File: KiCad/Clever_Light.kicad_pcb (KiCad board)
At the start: 2 copper layers, 50.8 x 50.8 mm, 18 parts, among them IC1 BTA08-600SWRG, J1 Screw_Terminal_01x02, J2 Screw_Terminal_01x02, J3 Screw_Terminal_01x02, J4 Screw_Terminal_01x02, J5 Conn_02x07_Odd_Even, Q1 SFH6156-3T, U1 MOC3063M

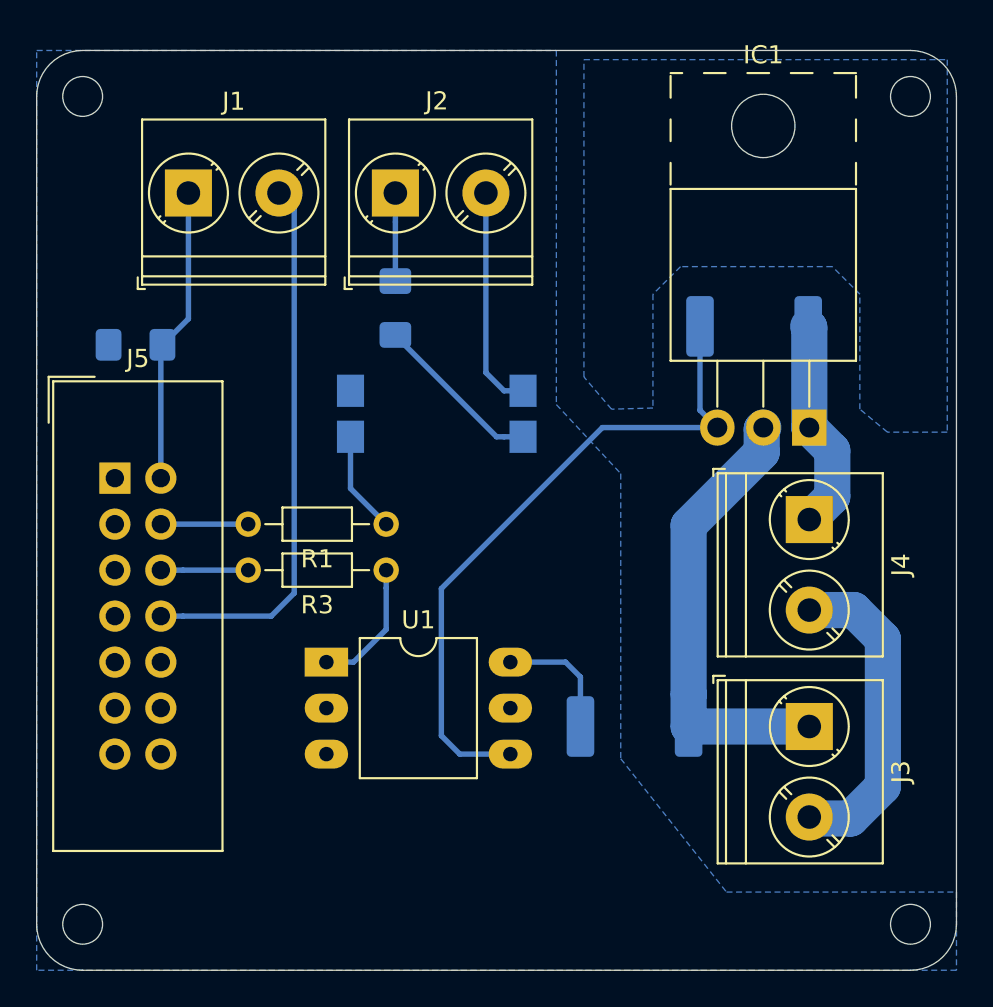
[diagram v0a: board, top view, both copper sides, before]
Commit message: небольшая оптимизация
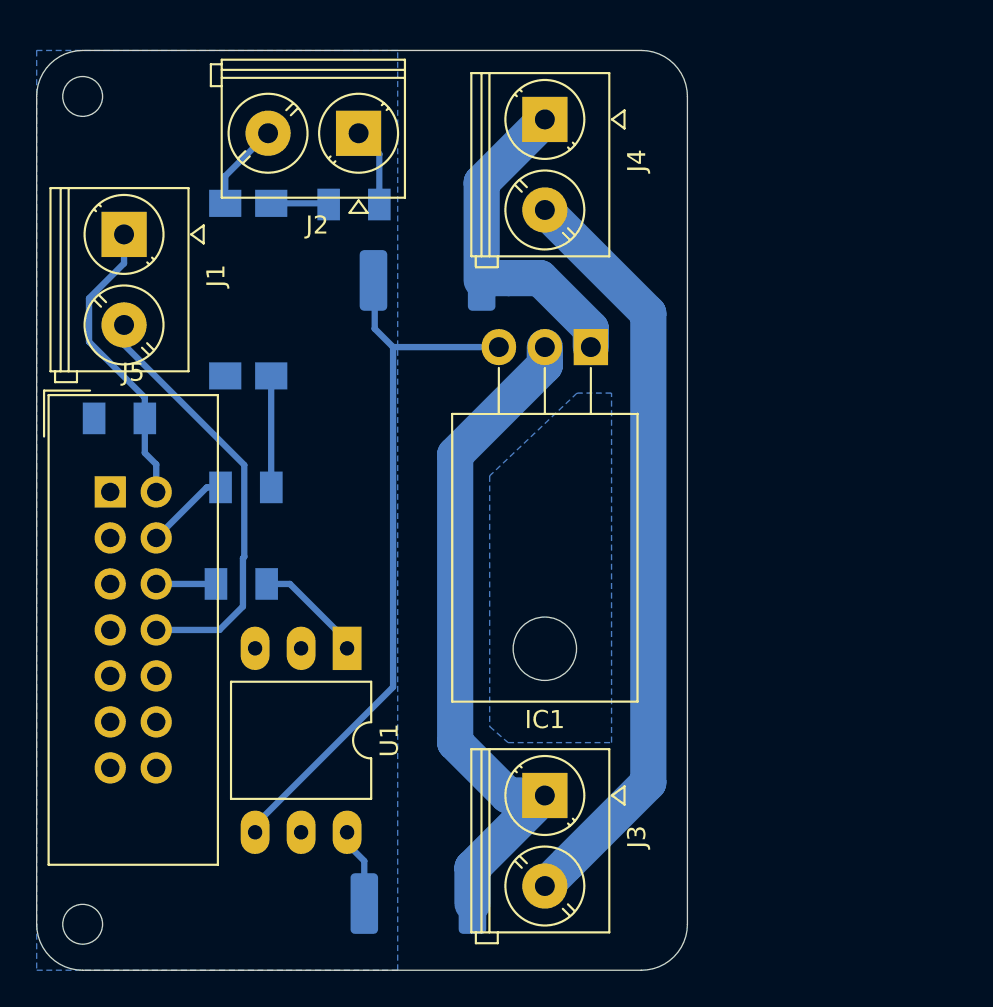
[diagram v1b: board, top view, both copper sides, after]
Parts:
- removed the REF** at (159.3, 93.2)
- removed the REF** at (159.3, 47.5)
- IC1: footprint Package_TO_SOT_THT:TO-220-3_Horizontal_TabUp -> Package_TO_SOT_THT:TO-220-3_Horizontal_TabDown
- J1, J2, J3, J4: footprint TerminalBlock_Phoenix:TerminalBlock_Phoenix_PT-1,5-2-5.0-H_1x02_P5.00mm_Horizontal -> TerminalBlock_Phoenix:TerminalBlock_KV301_1x02_P5.00mm_Horizontal
- R1, R3: footprint Resistor_THT:R_Axial_DIN0204_L3.6mm_D1.6mm_P7.62mm_Horizontal -> Resistor_SMD:R_1206_3216Metric; moved to B.Cu
- R2, R6: footprint Resistor_SMD:R_1206_3216Metric_Pad1.42x1.75mm_HandSolder -> Resistor_SMD:R_1206_3216Metric
- moved J4 26.5 mm to (139.1, 48.8)
- moved R5 18.2 mm to (132.6, 57.7)
- moved R4 15.4 mm to (132.1, 92.1)
- moved J3 15.1 mm to (139.1, 86.1)
- moved IC1 12.9 mm to (141.6, 61.3)
- moved Q1 12.5 mm to (122.7, 58.2), turned to 90 degrees
- moved R3 8.04 mm to (122.3, 74.4)
- moved R1 8.01 mm to (122.6, 69.1)
- moved R2 6.16 mm to (128.5, 53.5), turned to 180 degrees
- moved J1 4.23 mm to (115.8, 55.1), turned to 270 degrees
- moved R6 4.16 mm to (115.6, 65.3)
- moved J2 3.88 mm to (128.8, 49.5), turned to 180 degrees
- moved U1 1.37 mm to (128.1, 78.0), turned to 270 degrees
- moved J5 0.80 mm to (115.1, 69.3)
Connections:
- J5 pad 1: Net-(J5-Pad1) -> (no net)
- J5 pad 11: Net-(J5-Pad11) -> (no net)
- J5 pad 13: Net-(J5-Pad13) -> (no net)
- J5 pad 3: Net-(J5-Pad3) -> (no net)
- J5 pad 5: Net-(J5-Pad5) -> (no net)
- J5 pad 7: Net-(J5-Pad7) -> (no net)
- J5 pad 9: Net-(J5-Pad9) -> (no net)
- U1 pad 3: Net-(U1-Pad3) -> (no net)
- U1 pad 5: Net-(U1-Pad5) -> (no net)
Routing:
- net N: track 17.7 -> 42.1 mm
- net L: track 24.9 -> 37.7 mm
- net DIM-: track 12.4 -> 4.85 mm
- net Net-(Q1-Pad4): track 9.95 -> 3.20 mm
- net BUTTON2: track 30.3 -> 23.7 mm
- net LOAD: track 11.7 -> 17.9 mm
- net Net-(IC1-Pad3): track 37.3 -> 39.9 mm
- net Net-(R4-Pad2): track 6.94 -> 4.33 mm
- net ON: track 4.83 -> 3.30 mm
- net Net-(R3-Pad1): track 7.33 -> 6.15 mm
- net DIM+: track 5.41 -> 4.41 mm
- net Net-(Q1-Pad1): track 5.64 -> 6.16 mm
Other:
- board size 50.8 x 50.8 mm -> 35.9 x 50.8 mm
- net class Default: trace_width 0.25 -> 0.3
- net class Силовая: clearance 0.5 -> 0.51
- net class Слаботочная: clearance 0.5 -> 0.51; trace_width 0.3 -> 0.35
- rule trace_min: 0.2 -> 0.3
